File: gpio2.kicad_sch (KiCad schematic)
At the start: 2 parts, among them U27 RK3576

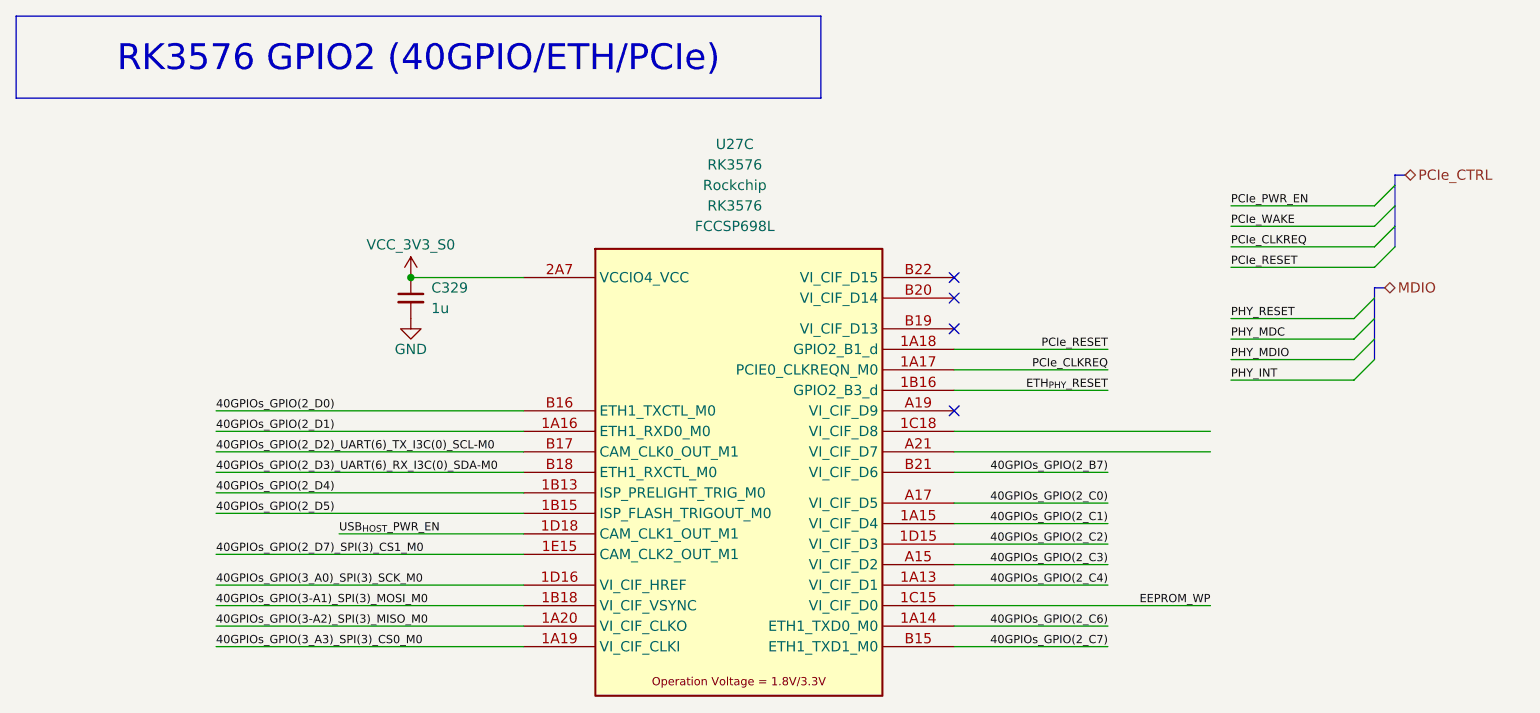
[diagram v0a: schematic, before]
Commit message: Add files via upload
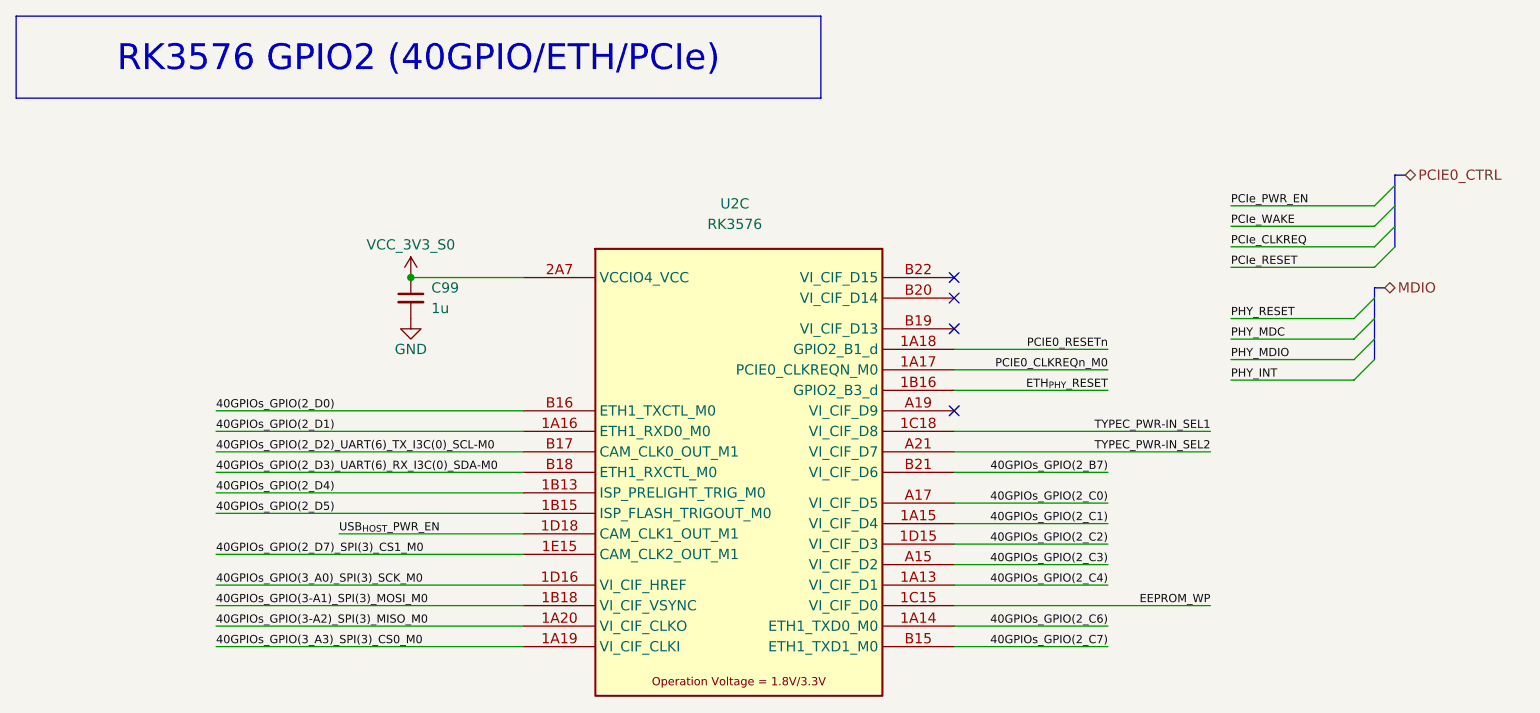
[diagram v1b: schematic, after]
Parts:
- renumbered C329 to C99, U27 to U2
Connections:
- net PCIe_CLKREQ: no longer U2.1A17 (VI_CIF_D11)
- net PCIe_RESET: no longer U2.1A18 (VI_CIF_D12)
- net TYPEC_PWR-IN_SEL1: now reaches U2.1C18 (VI_CIF_D8)
- net TYPEC_PWR-IN_SEL2: now reaches U2.A21 (VI_CIF_D7)
- new net PCIE0_CLKREQn_M0: U2.1A17 (VI_CIF_D11)
- new net PCIE0_RESETn: U2.1A18 (VI_CIF_D12)
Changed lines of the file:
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@@
 		)
 	)
-	(label "PCIe_RESET"
+	(label "PCIE0_RESETn"
 		(at 147.32 53.34 180)
 		(effects
@@
 		)
 	)
+	(label "TYPEC_PWR-IN_SEL1"
+		(at 160.02 63.5 180)
+		(effects
+			(font
+				(size 1.016 1.016)
+			)
+			(justify right bottom)
+		)
+	)
 	(label "PCIe_WAKE"
 		(at 162.56 38.1 0)
@@
 		)
 	)
-	(label "PCIe_CLKREQ"
+	(label "PCIE0_CLKREQn_M0"
 		(at 147.32 55.88 180)
+		(effects
+			(font
+				(size 1.016 1.016)
+			)
+			(justify right bottom)
+		)
+	)
+	(label "TYPEC_PWR-IN_SEL2"
+		(at 160.02 66.04 180)
 		(effects
 			(font
@@
 		)
 	)
-	(hierarchical_label "PCIe_CTRL"
+	(hierarchical_label "PCIE0_CTRL"
 		(shape bidirectional)
 		(at 184.15 31.75 0)
+		(fields_autoplaced yes)
 		(effects
 			(font
@@
 			)
 			(justify left)
+		)
+		(property "Netclass" "PCIE0_CTRL"
+			(at 184.15 33.02 0)
+			(hide yes)
+			(show_name no)
+			(do_not_autoplace no)
+			(effects
+				(font
+					(size 1.27 1.27)
+					(italic yes)
+				)
+				(justify left)
+			)
 		)
 	)
@@
 			)
 			(justify left)
+		)
+	)
+	(rule_area
+		(exclude_from_sim no)
+		(in_bom yes)
+		(on_board yes)
+		(dnp no)
+		(polyline
+			(pts
+				(xy 129.54 67.31) (xy 130.81 66.04) (xy 147.32 66.04) (xy 148.59 67.31) (xy 148.59 82.55) (xy 147.32 83.82)
+				(xy 130.81 83.82) (xy 129.54 82.55)
+			)
+			(stroke
+				(width 0)
+				(type dash)
+			)
+			(fill
+				(type none)
+			)
 		)
 	)
@@
 		(in_pos_files yes)
 		(dnp no)
-		(property "Reference" "U27"
-			(at 101.092 27.94 0)
+		(property "Reference" "U2"
+			(at 101.092 35.306 0)
 			(show_name no)
 			(do_not_autoplace no)
@@
 		)
 		(property "Value" "RK3576"
-			(at 101.092 30.48 0)
+			(at 101.092 37.846 0)
 			(show_name no)
 			(do_not_autoplace no)
@@
 		(property "Manf" "Rockchip"
 			(at 101.092 33.02 0)
+			(hide yes)
 			(show_name no)
 			(do_not_autoplace no)
@@
 		(property "MPN" "RK3576"
 			(at 101.092 35.56 0)
+			(hide yes)
 			(show_name no)
 			(do_not_autoplace no)
@@
 		(property "Package" "FCCSP698L"
 			(at 101.092 38.1 0)
+			(hide yes)
+			(show_name no)
+			(do_not_autoplace no)
+			(effects
+				(font
+					(size 1.27 1.27)
+				)
+			)
+		)
+		(property "Dielectric" ""
+			(at 101.6 68.58 0)
+			(hide yes)
+			(show_name no)
+			(do_not_autoplace no)
+			(effects
+				(font
+					(size 1.27 1.27)
+				)
+			)
+		)
+		(property "Voltage" ""
+			(at 101.6 68.58 0)
+			(hide yes)
+			(show_name no)
+			(do_not_autoplace no)
+			(effects
+				(font
+					(size 1.27 1.27)
+				)
+			)
+		)
+		(property "KLC_S3.3" ""
+			(at 101.6 68.58 0)
+			(hide yes)
+			(show_name no)
+			(do_not_autoplace no)
+			(effects
+				(font
+					(size 1.27 1.27)
+				)
+			)
+		)
+		(property "KLC_S4.1" ""
+			(at 101.6 68.58 0)
+			(hide yes)
+			(show_name no)
+			(do_not_autoplace no)
+			(effects
+				(font
+					(size 1.27 1.27)
+				)
+			)
+		)
+		(property "KLC_S5.1" ""
+			(at 101.6 68.58 0)
+			(hide yes)
 			(show_name no)
 			(do_not_autoplace no)
@@
 			(project "RK3576 SBC"
 				(path "/b79dbff4-0cad-4ff7-bec2-7c0e4f8b14d3/34f9b0cb-aeae-42b4-a2af-a0a79afcf392/90f1d3d6-11a1-4fbf-aa1e-f6ffe7a54522"
-					(reference "U27")
+					(reference "U2")
 					(unit 3)
 				)
@@
 		(in_pos_files yes)
 		(dnp no)
-		(property "Reference" "#PWR0425"
+		(property "Reference" "#PWR0136"
 			(at 60.96 48.26 0)
 			(hide yes)
@@
 			(project "RK3576 SBC"
 				(path "/b79dbff4-0cad-4ff7-bec2-7c0e4f8b14d3/34f9b0cb-aeae-42b4-a2af-a0a79afcf392/90f1d3d6-11a1-4fbf-aa1e-f6ffe7a54522"
-					(reference "#PWR0425")
+					(reference "#PWR0136")
 					(unit 1)
 				)
@@
 		(dnp no)
 		(fields_autoplaced yes)
-		(property "Reference" "C329"
+		(property "Reference" "C99"
 			(at 63.5 45.7262 0)
 			(show_name no)
@@
 		)
 		(property "Description" "Unpolarized capacitor, small symbol"
+			(at 60.96 46.99 0)
+			(hide yes)
+			(show_name no)
+			(do_not_autoplace no)
+			(effects
+				(font
+					(size 1.27 1.27)
+				)
+			)
+		)
+		(property "Dielectric" ""
+			(at 60.96 46.99 0)
+			(hide yes)
+			(show_name no)
+			(do_not_autoplace no)
+			(effects
+				(font
+					(size 1.27 1.27)
+				)
+			)
+		)
+		(property "Voltage" ""
+			(at 60.96 46.99 0)
+			(hide yes)
+			(show_name no)
+			(do_not_autoplace no)
+			(effects
+				(font
+					(size 1.27 1.27)
+				)
+			)
+		)
+		(property "KLC_S3.3" ""
+			(at 60.96 46.99 0)
+			(hide yes)
+			(show_name no)
+			(do_not_autoplace no)
+			(effects
+				(font
+					(size 1.27 1.27)
+				)
+			)
+		)
+		(property "KLC_S4.1" ""
+			(at 60.96 46.99 0)
+			(hide yes)
+			(show_name no)
+			(do_not_autoplace no)
+			(effects
+				(font
+					(size 1.27 1.27)
+				)
+			)
+		)
+		(property "KLC_S5.1" ""
 			(at 60.96 46.99 0)
 			(hide yes)
@@
 			(project "RK3576 SBC"
 				(path "/b79dbff4-0cad-4ff7-bec2-7c0e4f8b14d3/34f9b0cb-aeae-42b4-a2af-a0a79afcf392/90f1d3d6-11a1-4fbf-aa1e-f6ffe7a54522"
-					(reference "C329")
+					(reference "C99")
 					(unit 1)
 				)
@@
 		(in_pos_files yes)
 		(dnp no)
-		(property "Reference" "#PWR0426"
+		(property "Reference" "#PWR0137"
 			(at 60.96 55.88 0)
 			(hide yes)
@@
 			(project "RK3576 SBC"
 				(path "/b79dbff4-0cad-4ff7-bec2-7c0e4f8b14d3/34f9b0cb-aeae-42b4-a2af-a0a79afcf392/90f1d3d6-11a1-4fbf-aa1e-f6ffe7a54522"
-					(reference "#PWR0426")
+					(reference "#PWR0137")
 					(unit 1)
 				)
